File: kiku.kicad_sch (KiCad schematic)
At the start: 3 parts, among them J1 USB_C_Receptacle_USB2.0_16P, U1 ESP32-S3-WROOM-1, U2 Wio-sx1262-n

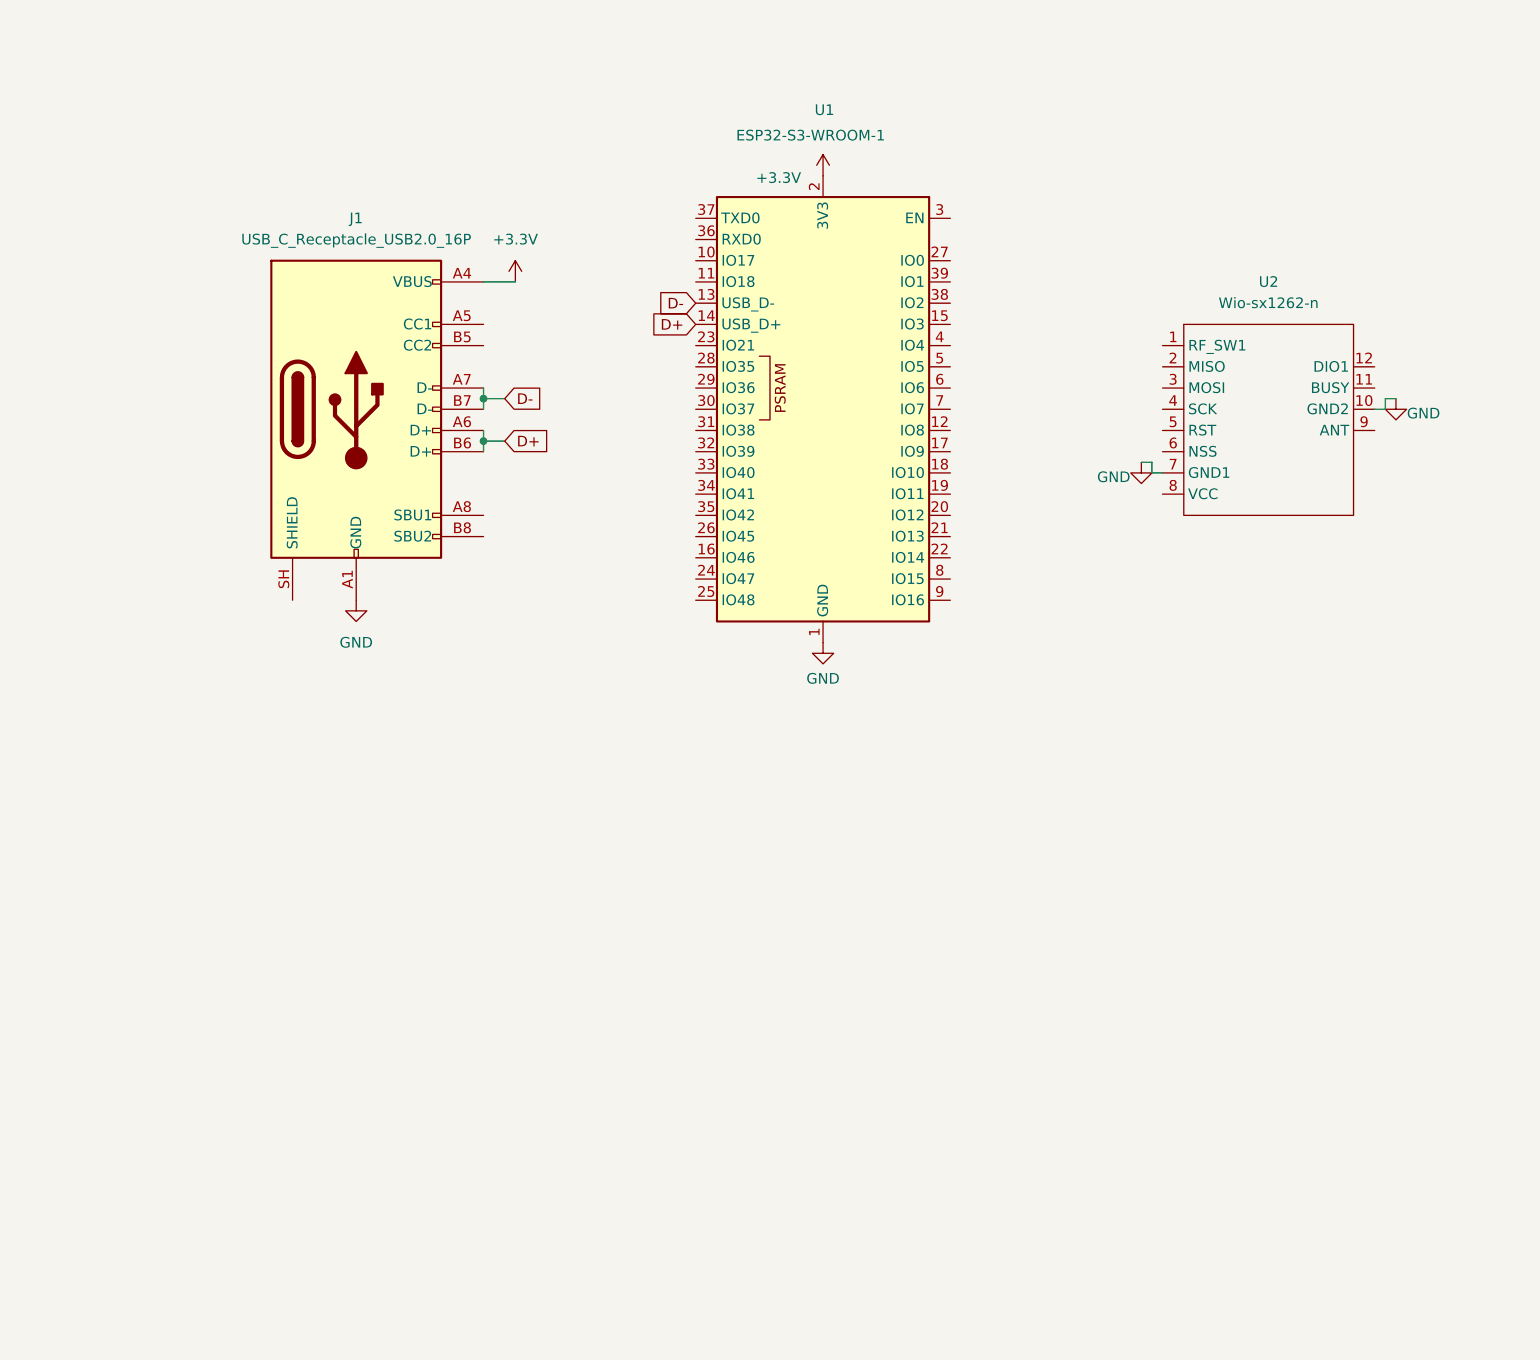
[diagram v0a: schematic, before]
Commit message: quite a bit of changes, still not finished with the schematic. havent committed in a while
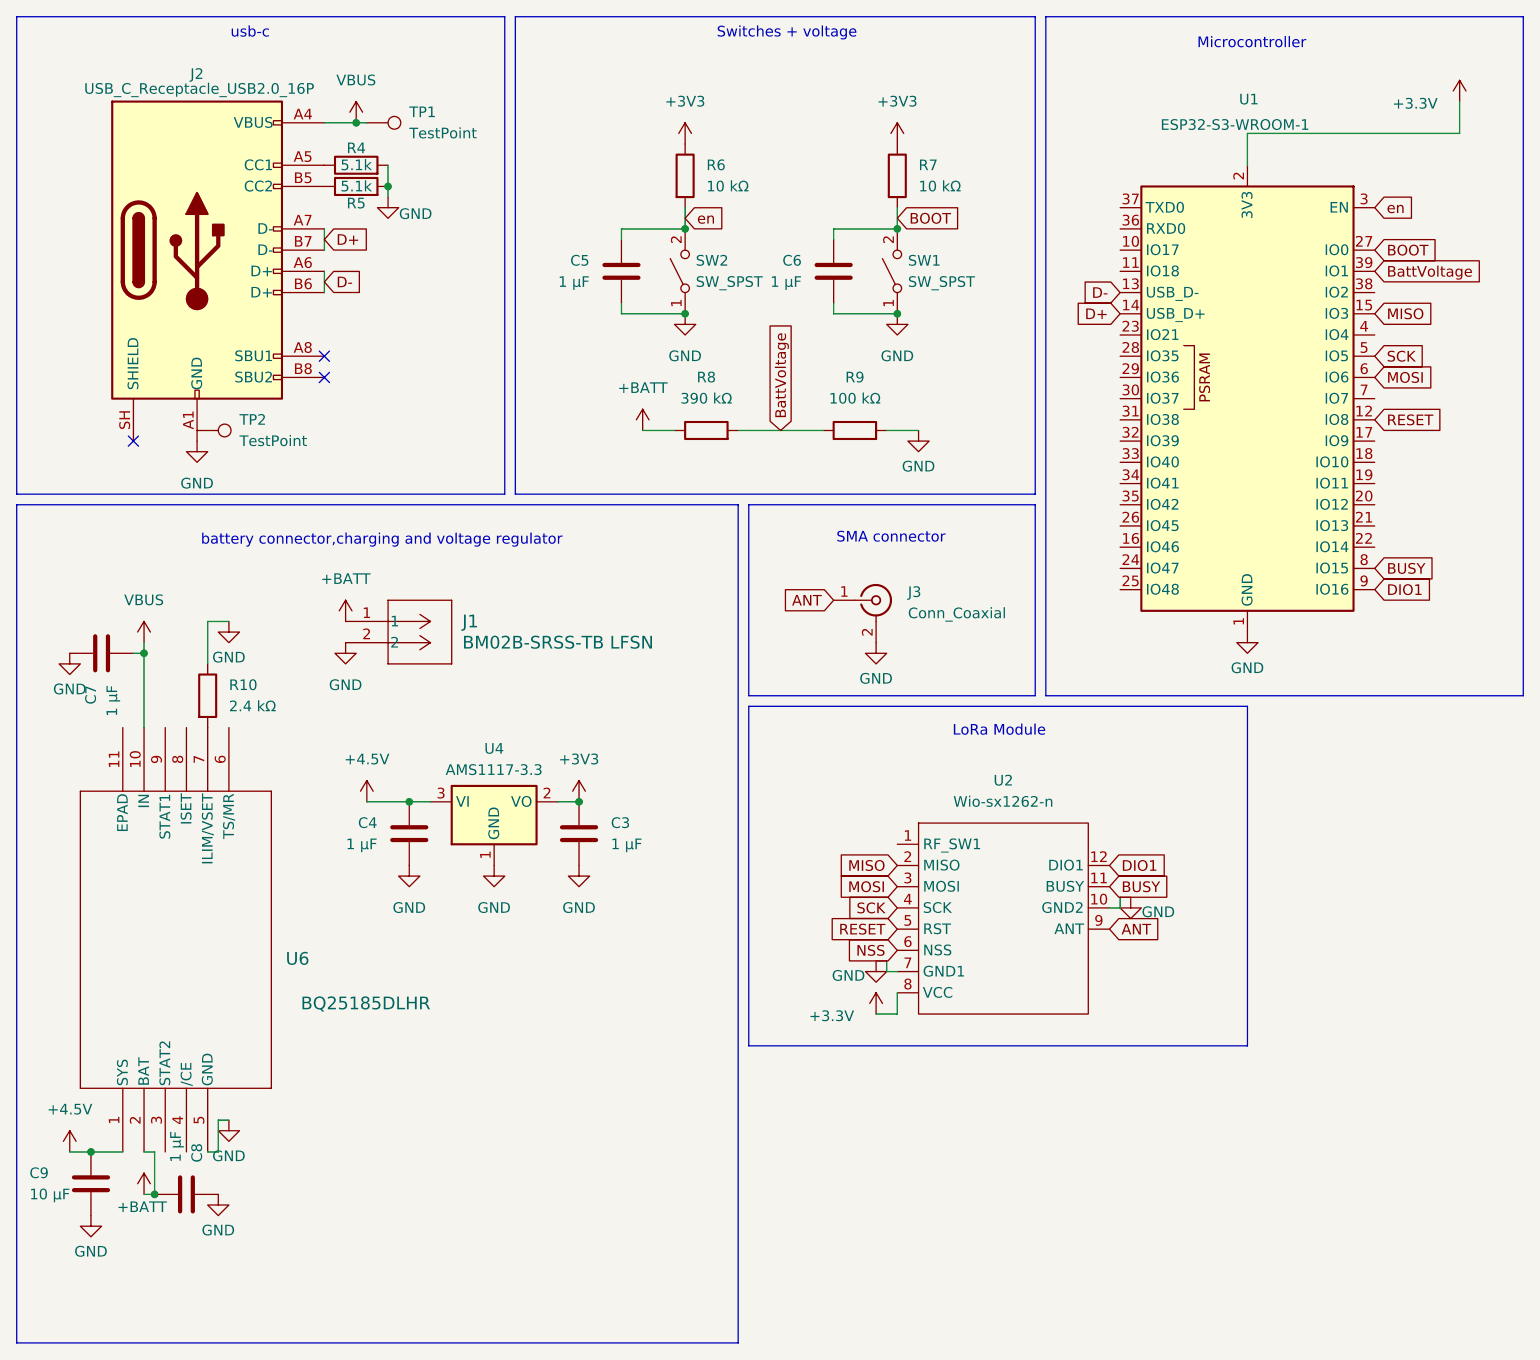
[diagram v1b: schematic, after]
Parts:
- removed J1: USB_C_Receptacle_USB2.0_16P, symbol Connector:USB_C_Receptacle_USB2.0_16P
- added C3, C4, C5, C6, C7, C8: 1 µF, Capacitor_SMD:C_0603_1608Metric, symbol Device:C
- added C9: 10 µF, Capacitor_SMD:C_0603_1608Metric, symbol Device:C
- added J1: BM02B-SRSS-TB LFSN, libraries:CONN_BM02B-SRSS-TB_JST, symbol libraries:BM02B-SRSS-TB_LFSN
- added J2: USB_C_Receptacle_USB2.0_16P, Connector_USB:USB_C_Receptacle_GCT_USB4105-xx-A_16P_TopMnt_Horizontal, symbol Connector:USB_C_Receptacle_USB2.0_16P
- added J3: Conn_Coaxial, Connector_Coaxial:SMA_Molex_73251-1153_EdgeMount_Horizontal, symbol Connector:Conn_Coaxial
- added R10: 2.4 kΩ, Resistor_SMD:R_0402_1005Metric, symbol Device:R
- added R4, R5: 5.1k, Resistor_SMD:R_0402_1005Metric, symbol Device:R
- added R6, R7: 10 kΩ, Resistor_SMD:R_0402_1005Metric, symbol Device:R
- added R8: 390 kΩ, Resistor_SMD:R_0402_1005Metric, symbol Device:R
- added R9: 100 kΩ, Resistor_SMD:R_0402_1005Metric, symbol Device:R
- added SW1, SW2: SW_SPST, Button_Switch_SMD:SW_SPST_B3U-1100P, symbol Switch:SW_SPST
- added TP1, TP2: TestPoint, TestPoint:TestPoint_Keystone_5010-5014_Multipurpose, symbol Connector:TestPoint
- added U4: AMS1117-3.3, Package_TO_SOT_SMD:SOT-223-3_TabPin2, symbol Regulator_Linear:AMS1117-3.3
- added U6: BQ25185DLHR, libraries:WSON10_DLH_TEX, symbol libraries:BQ25185DLHR
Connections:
- net +3.3V: now also U2.8 (VCC)
- net D+: now also J2.A7 (D-), J2.B7 (D-)
- net D-: now also J2.A6 (D+), J2.B6 (D+)
- net GND: now also C3.2, C4.2, C5.2, C6.2, C7.1, C8.1, C9.2, J1.2, J2.A1 (GND), J2.A12 (GND), J2.B1 (GND), J2.B12 (GND), J3.2 (Ext), R10.1, R4.2, R5.2, R9.2, SW1.1 (A), SW2.1 (A), U4.1 (GND), U6.5 (GND)
- net RESET: now reaches U1.12 (IO8)
- net RESET: now also U2.5 (RST)
- net MISO: now reaches U1.15 (IO3)
- net MISO: now also U2.2 (MISO)
- net BOOT: now reaches U1.27 (IO0)
- net BOOT: now also C6.1, R7.2, SW1.2 (B)
- net en: now reaches U1.3 (EN)
- net en: now also C5.1, R6.2, SW2.2 (B)
- net BattVoltage: now reaches U1.39 (IO1)
- net BattVoltage: now also R8.2, R9.1
- net SCK: now reaches U1.5 (IO5)
- net SCK: now also U2.4 (SCK)
- net MOSI: now reaches U1.6 (IO6)
- net MOSI: now also U2.3 (MOSI)
- net BUSY: now reaches U1.8 (IO15)
- net BUSY: now also U2.11 (BUSY)
- net DIO1: now reaches U1.9 (IO16)
- net DIO1: now also U2.12 (DIO1)
- net NSS: now reaches U2.6 (NSS)
- net ANT: now reaches U2.9 (ANT)
- net ANT: now also J3.1 (In)
- new net: J2.A5 (CC1), R4.1
- new net: R10.2, U6.7 (ILIM/VSET)
- new net: J2.B5 (CC2), R5.1
- new net +3V3: C3.1, R6.1, R7.1, U4.2 (VO)
- new net +4.5V: C4.1, C9.1, U4.3 (VI), U6.1 (SYS)
- new net +BATT: C8.2, J1.1, R8.1, U6.2 (BAT)
- new net VBUS: C7.2, J2.A4 (VBUS), J2.A9 (VBUS), J2.B4 (VBUS), J2.B9 (VBUS), TP1.1, U6.10 (IN)
- no-connect marks 0 -> 3
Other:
- note added: "LoRa Module"
- note added: "Microcontroller"
- note added: "SMA connector"
- note added: "Switches + voltage"
- note added: "battery connector,charging and voltage regulator"
- note added: "usb-c"
- moved on the sheet: U1, U2
